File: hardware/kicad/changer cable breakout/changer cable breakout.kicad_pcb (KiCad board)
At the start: 2 copper layers, 22 x 80 mm, 3 parts, among them J1 SDD-130J, J2 SDD-130J, J3 Test Points

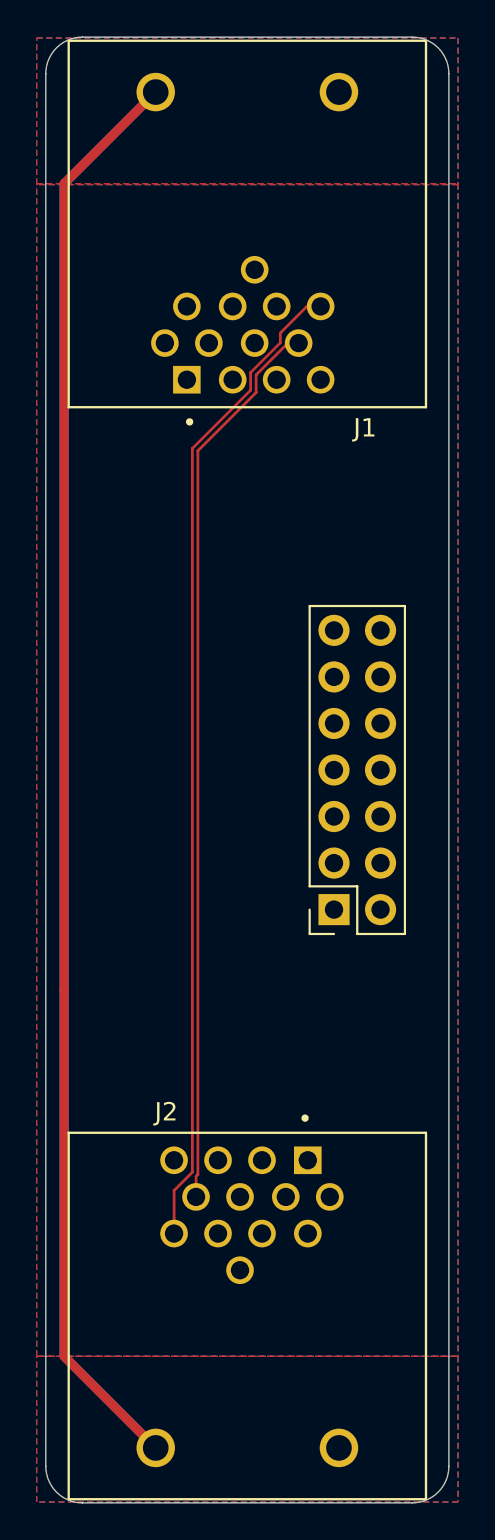
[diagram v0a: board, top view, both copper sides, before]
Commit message: finish breakout design
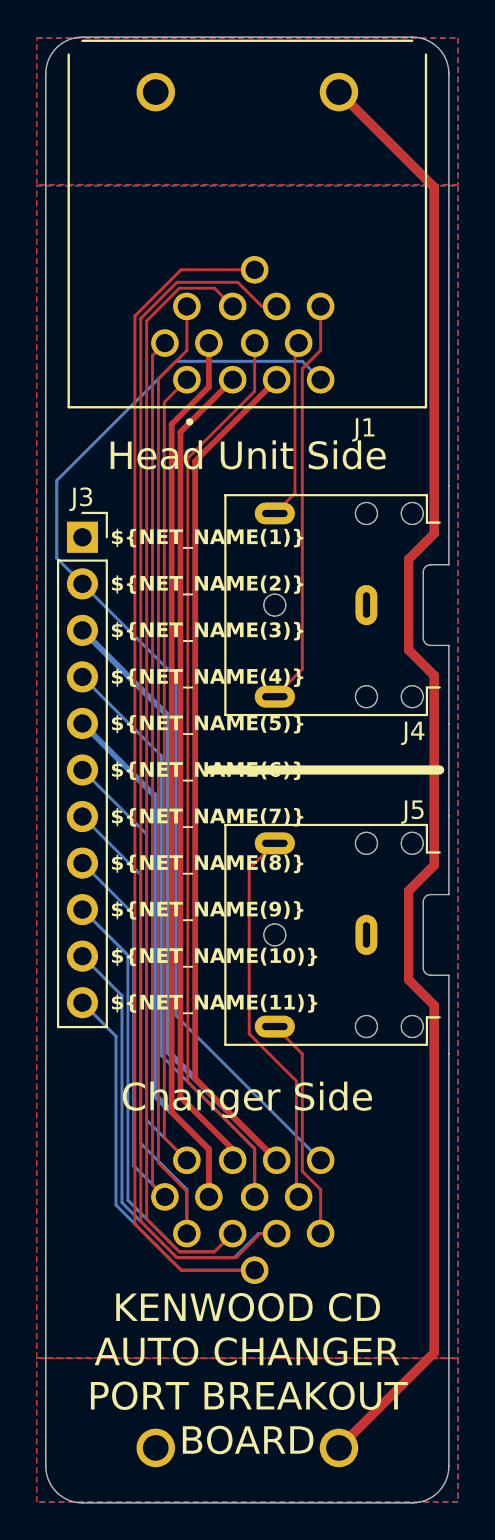
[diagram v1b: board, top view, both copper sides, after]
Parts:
- added J4: AudioJack3, Library:Jack_3.5mm_CUI_SJ1-3523N_Horizontal, F.Cu at (108.5, 95.0)
- added J5: AudioJack3, Library:Jack_3.5mm_CUI_SJ1-3523N_Horizontal, F.Cu at (108.5, 113.0)
- J2: moved to B.Cu
- J3: footprint Connector_PinSocket_2.54mm:PinSocket_2x07_P2.54mm_Vertical -> Library:PinSocket_1x11_P2.54mm_Vertical
- moved J3 15.0 mm to (93.0, 104.0), turned to 0 degrees
- turned J2 to 180 degrees
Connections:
- J1 pad 12: /L CH -> /L_ch_H
- J1 pad 8: /R_CH -> /R_ch_H
- J2 pad 12: /L CH -> /L_ch_C
- J2 pad 8: /R_CH -> /R_ch_C
- J3 pad 1: /~{REQ_H} -> /GND
- J3 pad 10: /DATA C -> /DATA H
- J3 pad 11: /DATA H -> /~{CLK}
- J3 pad 2: /GND -> /ON
- J3 pad 4: /ON -> /RESET
- J3 pad 5: /MUTE -> /D. GND
- J3 pad 6: /D. GND -> /~{REQ_H}
- J3 pad 7: /RESET -> /~{REQ_C}
- J3 pad 8: /R_CH -> /MUTE
- J3 pad 9: /~{REQ_C} -> /DATA C
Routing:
- net /DATA H: track 0.00 -> 91.4 mm
- net /~{CLK}: track 0.00 -> 85.6 mm
- net /DATA C: track 0.00 -> 84.9 mm
- net /RESET: track 0.00 -> 81.9 mm
- net /B.U.: track 0.00 -> 79.6 mm
- net /D. GND: track 0.00 -> 77.1 mm
- net /~{REQ_C}: track 0.00 -> 77.0 mm
- net /~{REQ_H}: track 0.00 -> 67.3 mm
- net /MUTE: track 0.00 -> 67.2 mm
- net /ON: track 0.00 -> 60.6 mm
- net /L CH: track 54.4 -> 0.00 mm
- net /R_CH: track 49.3 -> 0.00 mm
- net /GND: track 0.00 -> 45.0 mm
- net /L_ch_H: track 0.00 -> 22.3 mm
- net /R_ch_C: track 0.00 -> 21.0 mm
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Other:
- outline, holes or cut-outs redrawn
- board text added: "ALLEN KREAGER ${ISSUE_DATE} REV. ${REVISION}"
- board text added: "Changer Side"
- board text added: "Head Unit Side"
- board text added: "KENWOOD CD AUTO CHANGER PORT BREAKOUT BOARD"
- board text added: "https://github.com/akreager/cd_changer_emulator"
